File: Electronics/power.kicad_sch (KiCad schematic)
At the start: 50 parts, among them J1 USB_C_Receptacle_USB2.0, Q1 AON3419, Q2 AON3419, U2 STUSB4500QTR, U3 BQ25895RTW, U6 NCP186AMX330TAG, U7 MIC2250

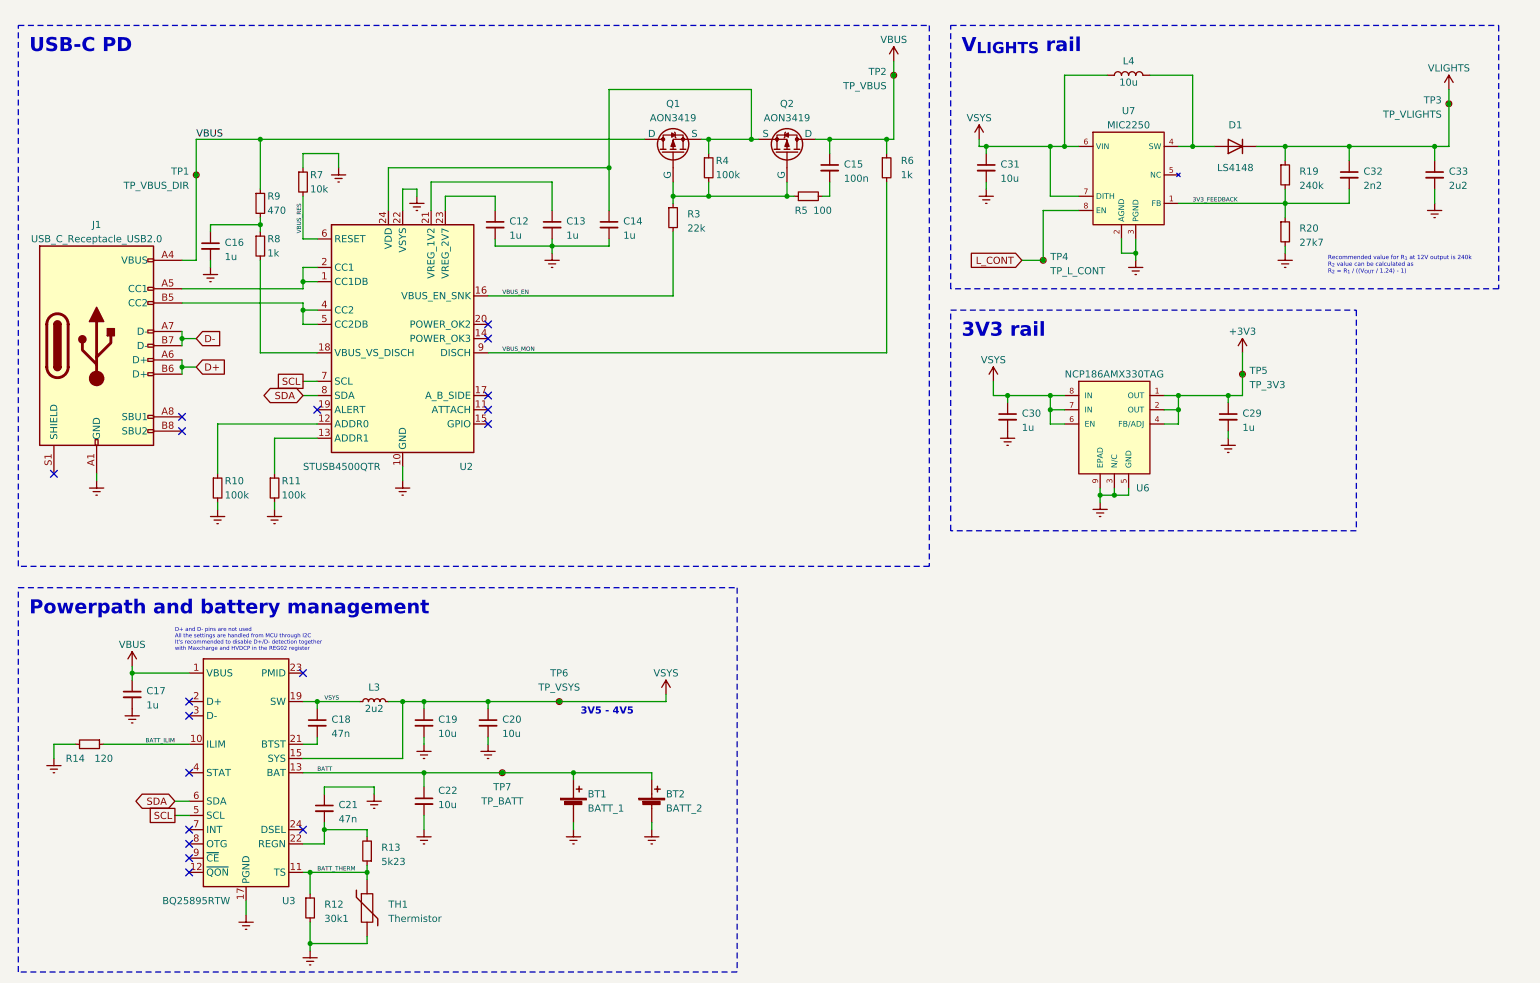
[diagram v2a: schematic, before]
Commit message: Power and lights update
Changed STUSB4500 + BQ25895 to MP2722. Changed Lights power supply, now it's split up to 3 LED drivers - KTD2801 as 10s1p. Added fuses to each battery. Added ESD protection. Fixed CHIP_EN pin name on ESP32-C3 and pull-up resistor on I2C lines.
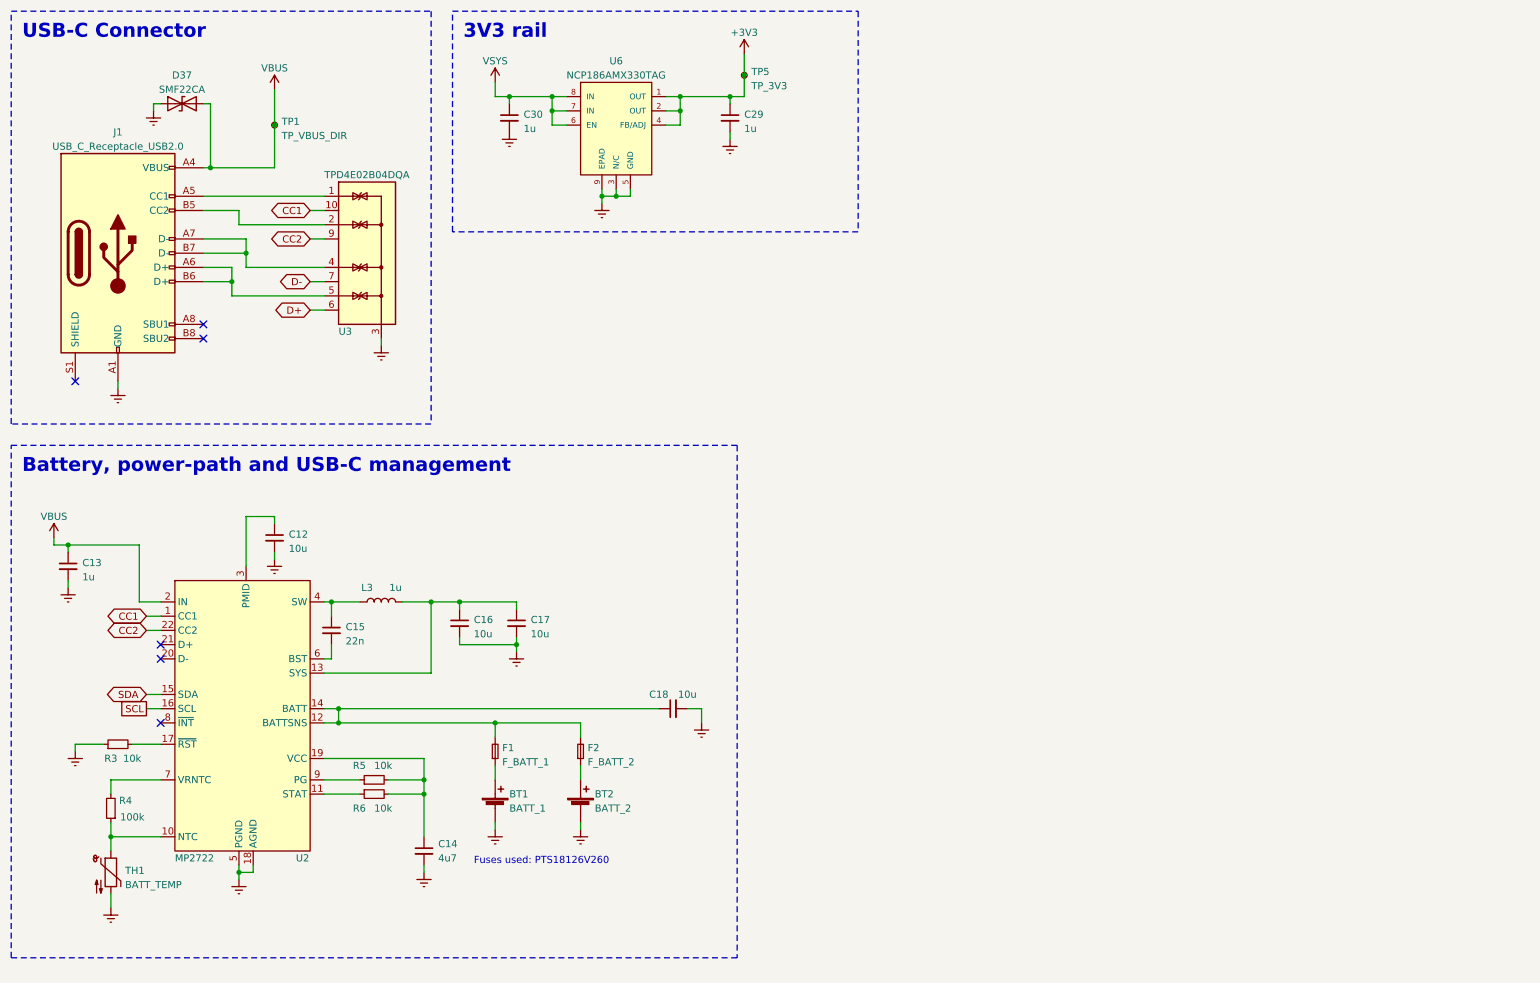
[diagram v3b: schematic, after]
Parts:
- removed C19, C20, C22, C31: 10u, symbol Device:C_Small
- removed C21: 47n, symbol Device:C_Small
- removed C32: 2n2, symbol Device:C_Small
- removed C33: 2u2, symbol Device:C_Small
- removed D1: LS4148, symbol Device:D
- removed L3: 2u2, symbol Device:L_Small
- removed L4: 10u, symbol Device:L
- removed Q1, Q2: AON3419, symbol Simulation_SPICE:PMOS
- removed R10, R11: 100k, symbol Device:R_Small
- removed R12: 30k1, symbol Device:R_Small
- removed R13: 5k23, symbol Device:R_Small
- removed R14: 120, symbol Device:R_Small
- removed R19: 240k, symbol Device:R_Small
- removed R20: 27k7, symbol Device:R_Small
- removed R7: 10k, symbol Device:R_Small
- removed R8: 1k, symbol Device:R_Small
- removed R9: 470, symbol Device:R_Small
- removed TH1: Thermistor, symbol Device:Thermistor
- removed TP2: TP_VBUS, symbol Connector:TestPoint_Small
- removed TP3: TP_VLIGHTS, symbol Connector:TestPoint_Small
- removed TP4: TP_L_CONT, symbol Connector:TestPoint_Small
- removed TP6: TP_VSYS, symbol Connector:TestPoint_Small
- removed TP7: TP_BATT, symbol Connector:TestPoint_Small
- removed U2: STUSB4500QTR, Package_DFN_QFN:QFN-24-1EP_4x4mm_P0.5mm_EP2.7x2.7mm, symbol Interface_USB:STUSB4500QTR
- removed U3: BQ25895RTW, Package_DFN_QFN:Texas_S-PWQFN-N24_EP2.7x2.7mm_ThermalVias, symbol Battery_Management:BQ25895RTW
- removed U7: MIC2250, Package_DFN_QFN:Micrel_MLF-8-1EP_2x2mm_P0.5mm_EP0.6x1.2mm, symbol Regulators_Switching:MIC2250
- added D37: SMF22CA, symbol Device:D_TVS
- added F1: F_BATT_1, symbol Device:Fuse_Small
- added F2: F_BATT_2, symbol Device:Fuse_Small
- added L3: 1u, symbol Device:L
- added TH1: BATT_TEMP, symbol Device:Thermistor_NTC
- added U2: MP2722, QFN-22:MP2722GRH0000Z, symbol Battery_ICs:MP2722
- added U3: TPD4E02B04DQA, Package_SON:USON-10_2.5x1.0mm_P0.5mm, symbol Power_Protection:TPD4E02B04DQA
- C12, C16, C17: value 1u -> 10u
- C14: value 1u -> 4u7
- C15: value 100n -> 22n
- C18: value 47n -> 10u
- R3: value 22k -> 10k
- R5: value 100 -> 10k
- R6: value 1k -> 10k
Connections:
- net VBUS_MON is gone; now on an unnamed net: R6.2
- net D+: now also U3.6 (NC); no longer J1.A6 (D+), J1.B6 (D+)
- net D-: now also U3.7 (NC); no longer J1.A7 (D-), J1.B7 (D-)
- net Earth: now also C18.2, R3.1, D37.1 (A1), TH1.2, U2.18 (AGND), U2.5 (PGND), U3.3 (G), U3.8 (G)
- net SCL: now also U2.16 (SCL)
- net SDA: now also U2.15 (SDA)
- net VBUS: now also C13.1, D37.2 (A2), U2.2 (IN); no longer C15.1, C17.1, R6.1
- net VSYS: no longer C18.1
- net at C12.1: now also U2.3 (PMID)
- net at J1.A5 (CC1): now also U3.1 (IO1)
- net at C14.1: now also R5.2, U2.19 (VCC); no longer R4.1
- net at J1.B5 (CC2): now also U3.2 (IO2)
- net at C15.2: now also U2.6 (BST); no longer R5.2
- net at C16.1: now also C17.1, L3.2, U2.13 (SYS)
- net BATT: no longer names the net of BT1.1 (+)
- net BATT: now also F1.1; no longer BT2.1 (+)
- net VBUS_EN: no longer names the net of R3.2
- net VBUS_EN: now also U2.17 (~{RST})
- new net: C18.1, F1.2, F2.2, U2.12 (BATTSNS), U2.14 (BATT)
- new net: R6.1, U2.11 (STAT)
- new net: R5.1, U2.9 (PG)
- new net: C15.1, L3.1, U2.4 (SW)
- new net: R4.1, TH1.1, U2.10 (NTC)
- new net: R4.2, U2.7 (VRNTC)
- new net: J1.A6 (D+), J1.B6 (D+), U3.5 (IO4)
- new net: J1.A7 (D-), J1.B7 (D-), U3.4 (IO3)
- new net: BT2.1 (+), F2.1
- new net CC1: U2.1 (CC1), U3.10 (NC)
- new net CC2: U2.22 (CC2), U3.9 (NC)
- no-connect marks 18 -> 6
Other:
- note added: "Fuses used: PTS18126V260"
- note removed: "3V5 - 4V5"
- note removed: "D+ and D- pins are not used All the settings are handled from MCU through I2C It's recommended to disable D+/D- detection together with Maxcharge and HVDCP in the REG02 register"
- note removed: "Recommended value for R_{1} at 12V output is 240k R_{2} value can be calculated as R_{2} = R_{1} / ((V_{OUT} / 1.24) - 1)"
- moved on the sheet: C29, C30, TP5, U6

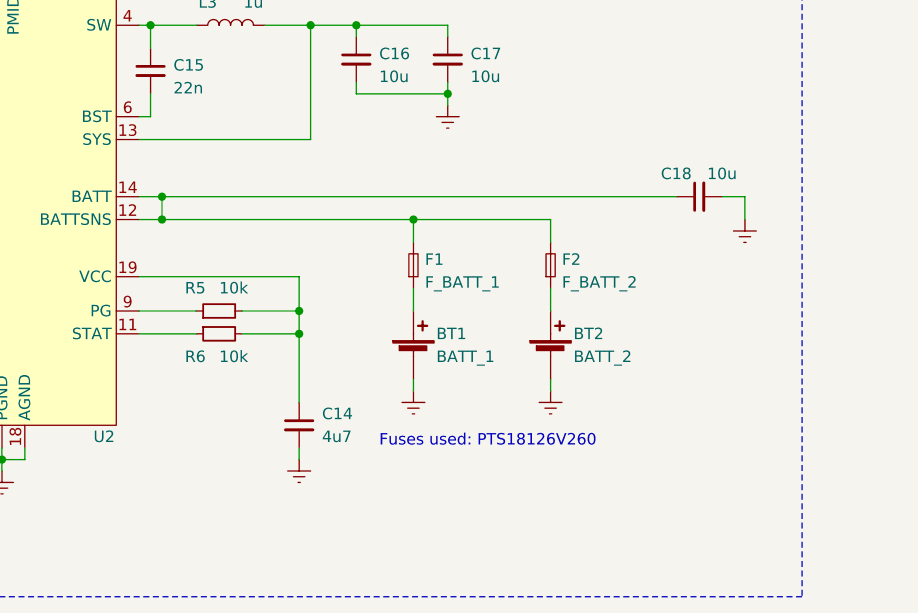
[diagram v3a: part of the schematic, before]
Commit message: Schematic update
Removed one battery, changed battery fuse to correct one. Fixed OLED connector
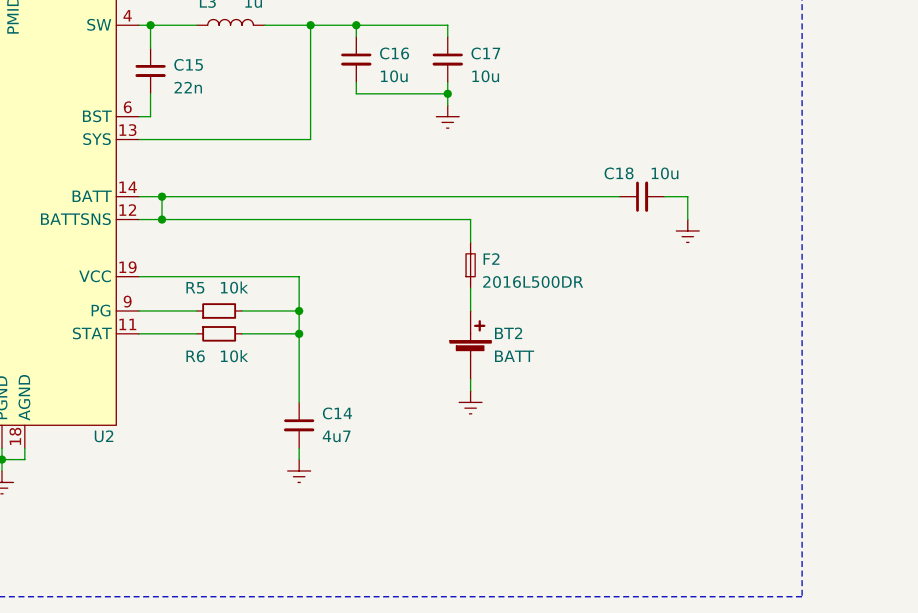
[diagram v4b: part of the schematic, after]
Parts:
- removed BT1: BATT_1, symbol Device:Battery_Cell
- removed F1: F_BATT_1, symbol Device:Fuse_Small
- BT2: value BATT_2 -> BATT
- F2: value F_BATT_2 -> 2016L500DR
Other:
- note removed: "Fuses used: PTS18126V260"
- moved on the sheet: BT2, C18, F2

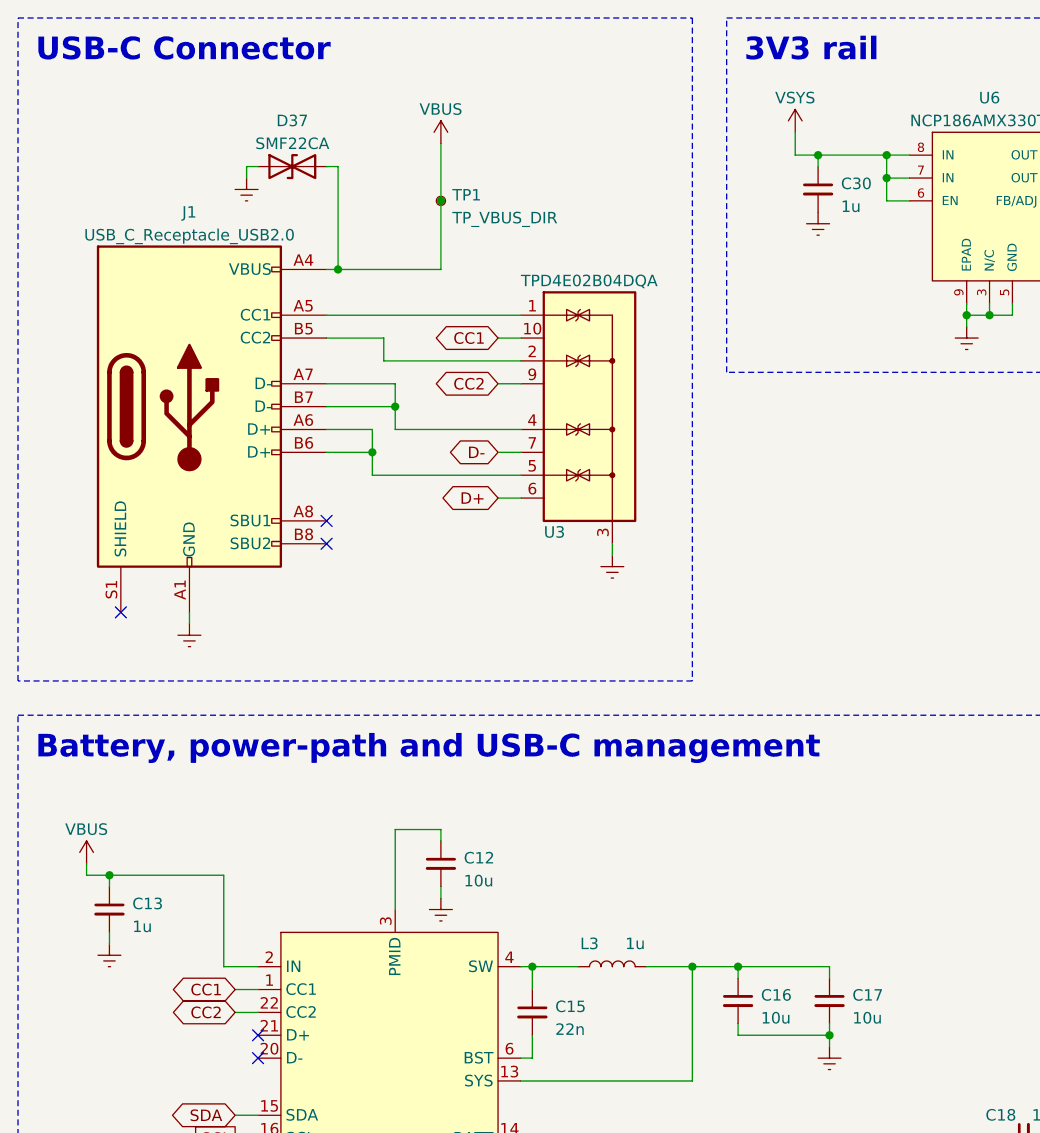
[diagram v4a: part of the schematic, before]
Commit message: PCB Layout mostly completed
Still have to finish LEDs layout on back side
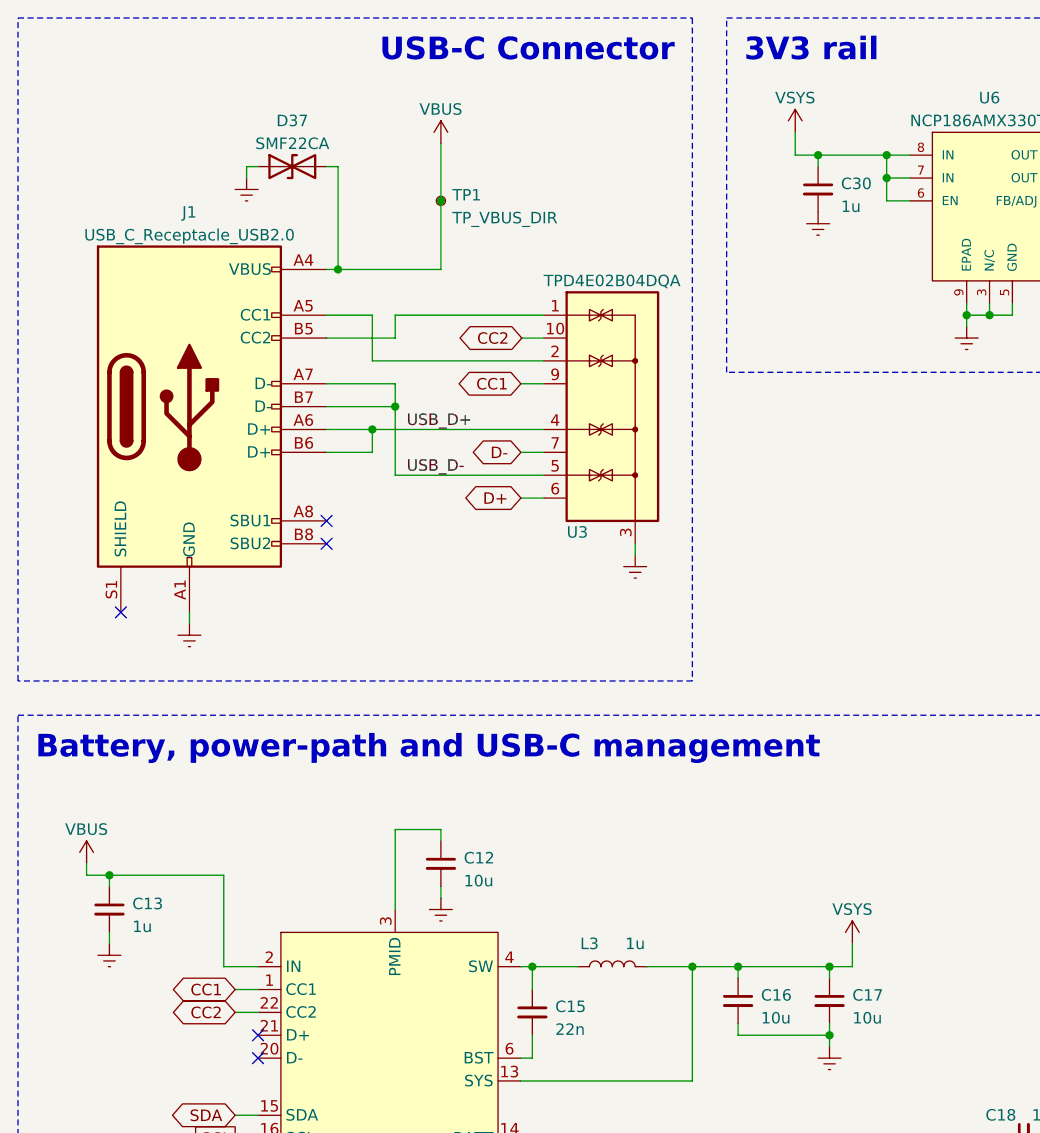
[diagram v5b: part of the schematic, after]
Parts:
- BT2: footprint (none) -> Connector_JST:JST_SH_BM02B-SRSS-TB_1x02-1MP_P1.00mm_Vertical
- C12, C16, C17, C18: footprint (none) -> Capacitor_SMD:C_0805_2012Metric
- C13, C14, C15, C29, C30: footprint (none) -> Capacitor_SMD:C_0603_1608Metric
- D37: footprint (none) -> Diode_SMD:D_SOD-123F
- F2: footprint (none) -> Fuse:Fuse_2010_5025Metric
- J1: footprint (none) -> Connector_USB:USB_C_Receptacle_Molex_105450-0101
- L3: footprint (none) -> Inductor_SMD:L_1210_3225Metric
- R3, R5, R6, TH1: footprint (none) -> Resistor_SMD:R_0402_1005Metric
- R4: footprint (none) -> Resistor_SMD:R_0603_1608Metric
- TP1, TP5: footprint (none) -> TestPoint:TestPoint_Pad_D2.0mm
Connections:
- net CC1: now also U3.9 (NC); no longer U3.10 (NC)
- net CC2: now also U3.10 (NC); no longer U3.9 (NC)
- net VSYS: now also C16.1, C17.1, L3.2, U2.13 (SYS)
- net at J1.A5 (CC1): now also U3.2 (IO2); no longer U3.1 (IO1)
- net USB_D+: now reaches J1.A6 (D+), J1.B6 (D+)
- net USB_D+: now also U3.4 (IO3); no longer U3.5 (IO4)
- net USB_D-: now reaches J1.A7 (D-), J1.B7 (D-)
- net USB_D-: now also U3.5 (IO4); no longer U3.4 (IO3)
- net at J1.B5 (CC2): now also U3.1 (IO1); no longer U3.2 (IO2)
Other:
- moved on the sheet: U3
